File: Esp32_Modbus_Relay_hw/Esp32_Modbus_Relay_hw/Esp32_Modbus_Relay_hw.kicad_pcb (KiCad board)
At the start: 2 copper layers, 121.6 x 86.8 mm, 0 parts

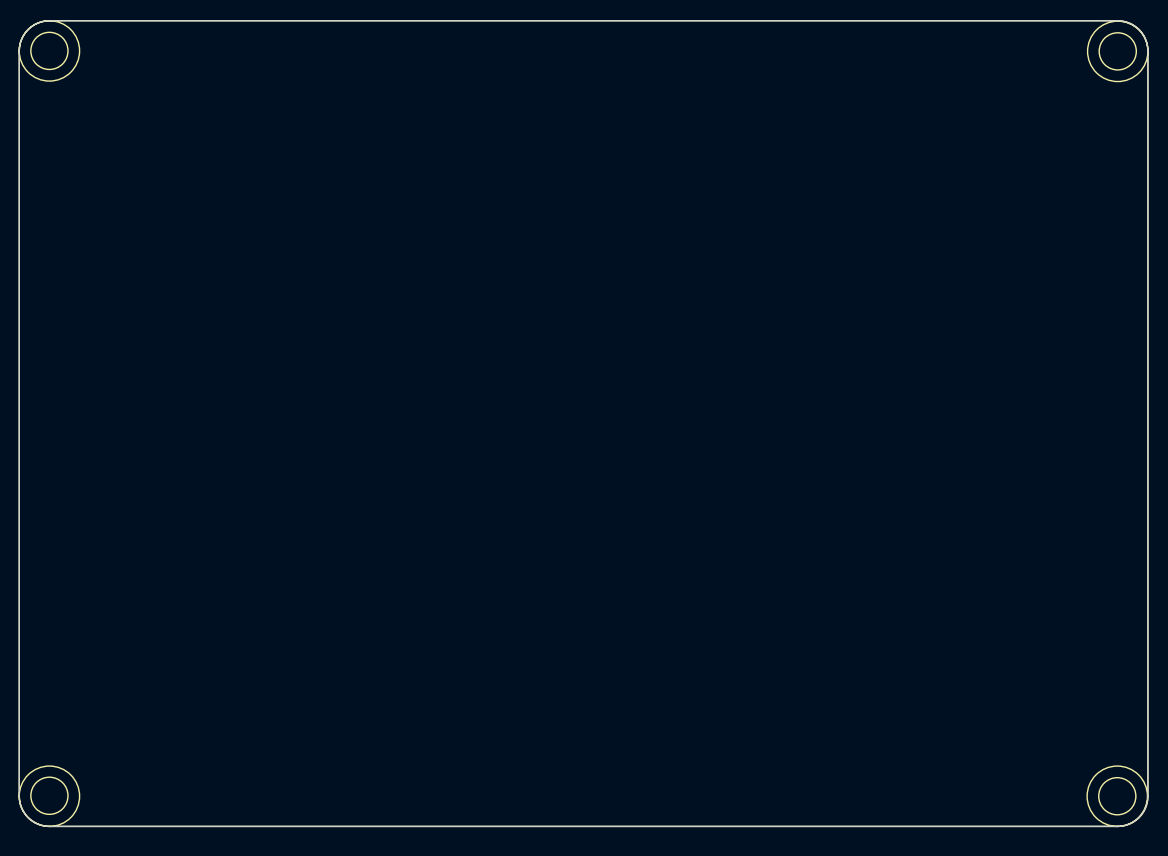
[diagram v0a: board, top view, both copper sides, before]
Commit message: Finish version 01
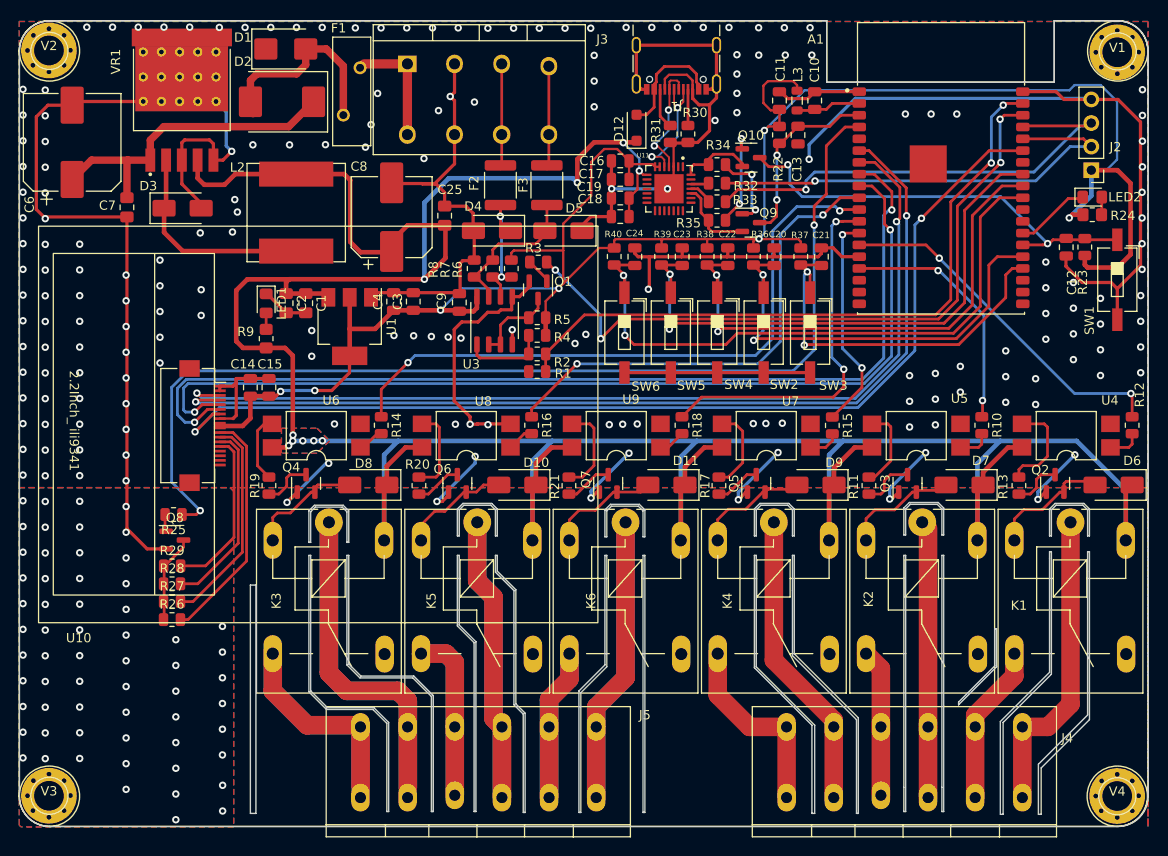
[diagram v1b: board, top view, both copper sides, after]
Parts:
- added A1: ESP32-WROVER-I, Lib_Hien:XCVR_ESP32-WROVER-I, F.Cu at (180.3, 57.9)
- added C1: 100nF, Capacitor_SMD:C_0805_2012Metric_Pad1.18x1.45mm_HandSolder, F.Cu at (111.9, 72.4)
- added C10: 100nF, Capacitor_SMD:C_0805_2012Metric, F.Cu at (166.7, 50.6)
- added C11: 1uF, Capacitor_SMD:C_0805_2012Metric, F.Cu at (162.9, 50.6)
- added C12: 100nF, Capacitor_SMD:C_0805_2012Metric, F.Cu at (193.8, 66.4)
- added C13: 100nF, Capacitor_SMD:C_0805_2012Metric, F.Cu at (164.9, 54.3)
- added C14: 10uF, Capacitor_SMD:C_0805_2012Metric, F.Cu at (105.9, 81.5)
- added C15: 100nF, Capacitor_SMD:C_0805_2012Metric, F.Cu at (107.9, 81.5)
- added C16: 100nF, Capacitor_SMD:C_0805_2012Metric, F.Cu at (145.8, 57.1)
- added C17: 100nF, Capacitor_SMD:C_0805_2012Metric, F.Cu at (145.8, 59.1)
- added C18: 100nF, Capacitor_SMD:C_0805_2012Metric, F.Cu at (145.8, 63.1)
- added C19: 100nF, Capacitor_SMD:C_0805_2012Metric, F.Cu at (145.8, 61.1)
- added C2: 10uF, Capacitor_SMD:C_0805_2012Metric_Pad1.18x1.45mm_HandSolder, F.Cu at (109.8, 72.4)
- added C20: 100nF, Capacitor_SMD:C_0805_2012Metric, F.Cu at (162.3, 67.4)
- added C21: 100nF, Capacitor_SMD:C_0805_2012Metric, F.Cu at (167.4, 67.4)
- added C22: 100nF, Capacitor_SMD:C_0805_2012Metric, F.Cu at (157.3, 67.4)
- added C23: 100nF, Capacitor_SMD:C_0805_2012Metric, F.Cu at (152.4, 67.4)
- added C24: 100nF, Capacitor_SMD:C_0805_2012Metric, F.Cu at (147.3, 67.4)
- added C25: 100nF, Capacitor_SMD:C_0805_2012Metric_Pad1.18x1.45mm_HandSolder, F.Cu at (126.8, 63.0)
- added C3: 10uF, Capacitor_SMD:C_0805_2012Metric, F.Cu at (123.5, 72.2)
- added C4: 100nF, Capacitor_SMD:C_0805_2012Metric, F.Cu at (121.3, 72.2)
- added C6: 470uF/25V, Capacitor_SMD:CP_Elec_10x10, F.Cu at (86.7, 55.1)
- added C7: 100nF, Capacitor_SMD:C_0805_2012Metric_Pad1.18x1.45mm_HandSolder, F.Cu at (92.6, 62.1)
- added C8: 220uF/25V, Capacitor_SMD:CP_Elec_8x10.5, F.Cu at (121.1, 63.2)
- added C9: 100nF, Capacitor_SMD:C_0805_2012Metric, F.Cu at (128.4, 72.3)
- added D1: TVS, Diode_SMD:D_SMB, F.Cu at (109.7, 45.0)
- added D10: 1N4148, Diode_SMD:D_SMA, F.Cu at (134.7, 92.0)
- added D11: 1N4148, Diode_SMD:D_SMA, F.Cu at (150.7, 92.0)
- added D12: 1N4007_T7, Diode_SMD:D_SOD-123F, F.Cu at (147.5, 53.5)
- added D2: ES3J_3A, Diode_SMD:D_SMC, F.Cu at (109.3, 50.7)
- added D3: 1N5820, Diode_SMD:D_SMA, F.Cu at (98.6, 62.2)
- added D4: D_TVS, Diode_SMD:D_SMA, F.Cu at (131.9, 64.6)
- added D5: D_TVS, Diode_SMD:D_SMA, F.Cu at (139.6, 64.6)
- added D6: 1N4148, Diode_SMD:D_SMA, F.Cu at (198.9, 92.0)
- added D7: 1N4148, Diode_SMD:D_SMA, F.Cu at (182.8, 92.0)
- added D8: 1N4148, Diode_SMD:D_SMA, F.Cu at (118.6, 92.0)
- added D9: 1N4148, Diode_SMD:D_SMA, F.Cu at (166.8, 92.0)
- added F1: UF300_3A, Fuse:Fuse_BelFuse_0ZRE0033FF_L11.4mm_W3.8mm, F.Cu at (117.7, 47.1)
- added F2: Fuse, Lib_Hien:Fuse_SMD_1812, F.Cu at (133.2, 59.6)
- added F3: Fuse, Lib_Hien:Fuse_SMD_1812, F.Cu at (138.2, 59.6)
- added J1: USB_C_Receptacle_USB2.0, Connector_USB:USB_C_Receptacle_GCT_USB4105-xx-A_16P_TopMnt_Horizontal, F.Cu at (151.8, 45.7)
- added J2: UART0_EXT, Connector_PinHeader_2.54mm:PinHeader_1x04_P2.54mm_Vertical, F.Cu at (196.5, 58.1)
- added J3: header input, Lib_Hien:KF142_4P_5.08, F.Cu at (122.8, 46.6)
- added J4: Conn_01x06_Pin, Lib_Hien:KF142_6P_5.08, F.Cu at (192.8, 115.9)
- added J5: Conn_01x06_Pin, Lib_Hien:KF142_6P_5.08, F.Cu at (146.8, 115.9)
- added K1: SRA-5VDC-CL, Relay_THT:Relay_SPDT_SANYOU_SRD_Series_Form_C, F.Cu at (194.3, 96.0)
- added K2: SRA-5VDC-CL, Relay_THT:Relay_SPDT_SANYOU_SRD_Series_Form_C, F.Cu at (178.3, 96.0)
- added K3: SRA-5VDC-CL, Relay_THT:Relay_SPDT_SANYOU_SRD_Series_Form_C, F.Cu at (114.4, 96.0)
- added K4: SRA-5VDC-CL, Relay_THT:Relay_SPDT_SANYOU_SRD_Series_Form_C, F.Cu at (162.3, 96.0)
- added K5: SRA-5VDC-CL, Relay_THT:Relay_SPDT_SANYOU_SRD_Series_Form_C, F.Cu at (130.3, 96.0)
- added K6: SRA-5VDC-CL, Relay_THT:Relay_SPDT_SANYOU_SRD_Series_Form_C, F.Cu at (146.3, 96.0)
- added L2: 33uH_2.9A, Lib_Hien:L_10x10, F.Cu at (110.5, 62.6)
- added L3: 10uH, Inductor_SMD:L_0805_2012Metric, F.Cu at (164.8, 50.6)
- added LED1: RED, LED_SMD:LED_0805_2012Metric_Pad1.15x1.40mm_HandSolder, F.Cu at (107.6, 72.5)
- added LED2: RED, LED_SMD:LED_0805_2012Metric_Pad1.15x1.40mm_HandSolder, F.Cu at (196.6, 61.0)
- added Q1: 2SC1815-HF, Package_TO_SOT_SMD:SOT-23, F.Cu at (136.9, 71.0)
- added Q10: S8050, Package_TO_SOT_SMD:SOT-23, F.Cu at (159.8, 56.8)
- added Q2: 2SC1815/HF, Package_TO_SOT_SMD:SOT-23, F.Cu at (192.6, 91.8)
- added Q3: 2SC1815/HF, Package_TO_SOT_SMD:SOT-23, F.Cu at (176.7, 91.8)
- added Q4: 2SC1815/HF, Package_TO_SOT_SMD:SOT-23, F.Cu at (111.9, 91.8)
- added Q5: 2SC1815/HF, Package_TO_SOT_SMD:SOT-23, F.Cu at (160.4, 91.8)
- added Q6: 2SC1815/HF, Package_TO_SOT_SMD:SOT-23, F.Cu at (128.2, 91.8)
- added Q7: 2SC1815/HF, Package_TO_SOT_SMD:SOT-23, F.Cu at (144.4, 91.8)
- added Q8: 2SC1815-HF, Package_TO_SOT_SMD:SOT-23, F.Cu at (97.8, 98.0)
- added Q9: S8050, Package_TO_SOT_SMD:SOT-23, F.Cu at (159.8, 63.8)
- added R1: 10K, Resistor_SMD:R_0805_2012Metric, F.Cu at (136.8, 79.8)
- added R10: 330R, Resistor_SMD:R_0805_2012Metric, F.Cu at (184.7, 85.6)
- added R11: 1k, Resistor_SMD:R_0805_2012Metric, F.Cu at (172.5, 92.1)
- added R12: 330R, Resistor_SMD:R_0805_2012Metric, F.Cu at (200.9, 85.6)
- added R13: 1k, Resistor_SMD:R_0805_2012Metric, F.Cu at (188.7, 92.1)
- added R14: 330R, Resistor_SMD:R_0805_2012Metric, F.Cu at (120.0, 85.6)
- added R15: 330R, Resistor_SMD:R_0805_2012Metric, F.Cu at (168.6, 85.6)
- added R16: 330R, Resistor_SMD:R_0805_2012Metric, F.Cu at (136.2, 85.6)
- added R17: 1k, Resistor_SMD:R_0805_2012Metric, F.Cu at (156.4, 92.1)
- added R18: 330R, Resistor_SMD:R_0805_2012Metric, F.Cu at (152.4, 85.6)
- added R19: 1k, Resistor_SMD:R_0805_2012Metric, F.Cu at (107.9, 92.1)
- added R2: 4.7K, Resistor_SMD:R_0805_2012Metric, F.Cu at (136.8, 77.9)
- added R20: 1k, Resistor_SMD:R_0805_2012Metric, F.Cu at (124.1, 92.1)
- added R21: 1k, Resistor_SMD:R_0805_2012Metric, F.Cu at (140.2, 92.1)
- added R22: 10K, Resistor_SMD:R_0805_2012Metric, F.Cu at (162.9, 54.3)
- added R23: 10K, Resistor_SMD:R_0805_2012Metric, F.Cu at (195.8, 66.4)
- added R24: 1K, Resistor_SMD:R_0805_2012Metric_Pad1.20x1.40mm_HandSolder, F.Cu at (196.6, 62.9)
- added R25: 2.2K, Resistor_SMD:R_0805_2012Metric, F.Cu at (97.6, 95.2)
- added R26: 220R, Resistor_SMD:R_0805_2012Metric, F.Cu at (97.5, 106.5)
- added R27: 220R, Resistor_SMD:R_0805_2012Metric, F.Cu at (97.5, 104.6)
- added R28: 220R, Resistor_SMD:R_0805_2012Metric, F.Cu at (97.5, 102.7)
- added R29: 220R, Resistor_SMD:R_0805_2012Metric, F.Cu at (97.5, 100.7)
- added R3: 2.2K, Resistor_SMD:R_0805_2012Metric, F.Cu at (136.9, 68.0)
- added R30: 5.1K, Resistor_SMD:R_0805_2012Metric, F.Cu at (153.0, 54.2)
- added R31: 5.1K, Resistor_SMD:R_0805_2012Metric, F.Cu at (151.1, 54.2)
- added R32: 470R, Resistor_SMD:R_0805_2012Metric, F.Cu at (156.2, 59.5)
- added R33: 470R, Resistor_SMD:R_0805_2012Metric, F.Cu at (156.2, 61.5)
- added R34: 10k, Resistor_SMD:R_0805_2012Metric, F.Cu at (156.2, 57.5)
- added R35: 10k, Resistor_SMD:R_0805_2012Metric, F.Cu at (156.2, 63.5)
- added R36: 10K, Resistor_SMD:R_0805_2012Metric, F.Cu at (160.1, 67.4)
- added R37: 10K, Resistor_SMD:R_0805_2012Metric, F.Cu at (165.2, 67.4)
- added R38: 10K, Resistor_SMD:R_0805_2012Metric, F.Cu at (155.1, 67.4)
- added R39: 10K, Resistor_SMD:R_0805_2012Metric, F.Cu at (150.2, 67.4)
- added R4: 10K, Resistor_SMD:R_0805_2012Metric, F.Cu at (136.8, 75.9)
- added R40: 10K, Resistor_SMD:R_0805_2012Metric, F.Cu at (145.1, 67.4)
- added R5: 10K, Resistor_SMD:R_0805_2012Metric, F.Cu at (136.8, 74.0)
- added R6: 4.7K, Resistor_SMD:R_0805_2012Metric, F.Cu at (134.0, 68.7)
- added R7: 120R, Resistor_SMD:R_0805_2012Metric, F.Cu at (132.0, 68.7)
- added R8: 4.7K, Resistor_SMD:R_0805_2012Metric, F.Cu at (130.0, 68.7)
- added R9: 2.2K, Resistor_SMD:R_0805_2012Metric_Pad1.20x1.40mm_HandSolder, F.Cu at (107.6, 76.2)
- added SW1: SW_Push, Button_Switch_SMD:SW_DIP_SPSTx01_Slide_6.7x4.1mm_W8.61mm_P2.54mm_LowProfile, F.Cu at (199.3, 69.9)
- added SW2: SW_Push, Button_Switch_SMD:SW_DIP_SPSTx01_Slide_6.7x4.1mm_W8.61mm_P2.54mm_LowProfile, F.Cu at (161.2, 75.6)
- added SW3: SW_Push, Button_Switch_SMD:SW_DIP_SPSTx01_Slide_6.7x4.1mm_W8.61mm_P2.54mm_LowProfile, F.Cu at (166.2, 75.6)
- added SW4: SW_Push, Button_Switch_SMD:SW_DIP_SPSTx01_Slide_6.7x4.1mm_W8.61mm_P2.54mm_LowProfile, F.Cu at (156.2, 75.6)
- added SW5: SW_Push, Button_Switch_SMD:SW_DIP_SPSTx01_Slide_6.7x4.1mm_W8.61mm_P2.54mm_LowProfile, F.Cu at (151.2, 75.6)
- added SW6: SW_Push, Button_Switch_SMD:SW_DIP_SPSTx01_Slide_6.7x4.1mm_W8.61mm_P2.54mm_LowProfile, F.Cu at (146.2, 75.6)
- added U1: AMS1117-3.3, Package_TO_SOT_SMD:SOT-223-3_TabPin2, F.Cu at (116.6, 75.0)
- added U10: 2.2inch_TFT_ILI9341_SPI, Lib_Hien:TFT_ILI9341_2.2INCH, F.Cu at (143.3, 64.1)
- added U11: CP2102-GM, Lib_Hien:CP2102, F.Cu at (151.0, 60.1)
- added U3: MAX485, Package_SO:SO-8_3.9x4.9mm_P1.27mm, F.Cu at (132.2, 74.3)
- added U4: PC817, Package_DIP:SMDIP-4_W9.53mm, F.Cu at (193.8, 86.7)
- added U5: PC817, Package_DIP:SMDIP-4_W9.53mm, F.Cu at (177.6, 86.7)
- added U6: PC817, Package_DIP:SMDIP-4_W9.53mm, F.Cu at (113.0, 86.7)
- added U7: PC817, Package_DIP:SMDIP-4_W9.53mm, F.Cu at (161.5, 86.7)
- added U8: PC817, Package_DIP:SMDIP-4_W9.53mm, F.Cu at (129.2, 86.7)
- added U9: PC817, Package_DIP:SMDIP-4_W9.53mm, F.Cu at (145.3, 86.7)
- added V1: Vit, Lib_Hien:Vit, F.Cu at (199.3, 45.4)
- added V2: Vit, Lib_Hien:Vit, F.Cu at (84.2, 45.2)
- added V3: Vit, Lib_Hien:Vit, F.Cu at (84.2, 125.5)
- added V4: Vit, Lib_Hien:Vit, F.Cu at (199.3, 125.5)
- added VR1: LM2596S-ADJ, Lib_Hien:LM2596S-ADJ, F.Cu at (98.5, 50.5)
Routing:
- net GND: track 0.00 -> 434.1 mm, vias 0 -> 249
- net +5V: track 0.00 -> 366.6 mm, vias 0 -> 10
- net +3.3V: track 0.00 -> 227.1 mm, vias 0 -> 7
- net /LCD_BL: track 0.00 -> 114.5 mm, vias 0 -> 2
- net /LCD_MISO: track 0.00 -> 113.1 mm, vias 0 -> 2
- net /LCD_MOSI: track 0.00 -> 108.5 mm, vias 0 -> 2
- net /LCD_DC: track 0.00 -> 106.1 mm, vias 0 -> 2
- net /LCD_CS0: track 0.00 -> 105.0 mm, vias 0 -> 2
- net /LCD_SCL: track 0.00 -> 104.2 mm, vias 0 -> 2
- net /TXD1: track 0.00 -> 75.0 mm, vias 0 -> 4
- net /RXD1: track 0.00 -> 73.6 mm, vias 0 -> 2
- net /COM6: track 0.00 -> 71.0 mm
- net /DO6: track 0.00 -> 69.6 mm, vias 0 -> 2
- net /OK: track 0.00 -> 67.7 mm, vias 0 -> 2
- net /RIGHT: track 0.00 -> 62.4 mm, vias 0 -> 2
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- added copper zone on B.Cu, net +5V
- added copper zone on F.Cu, net +5V
- added copper zone on B.Cu, net GND
- added copper zone on F.Cu, net GND
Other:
- outline, holes or cut-outs redrawn
